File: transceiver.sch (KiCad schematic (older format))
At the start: 1 part, among them U3 CC1200

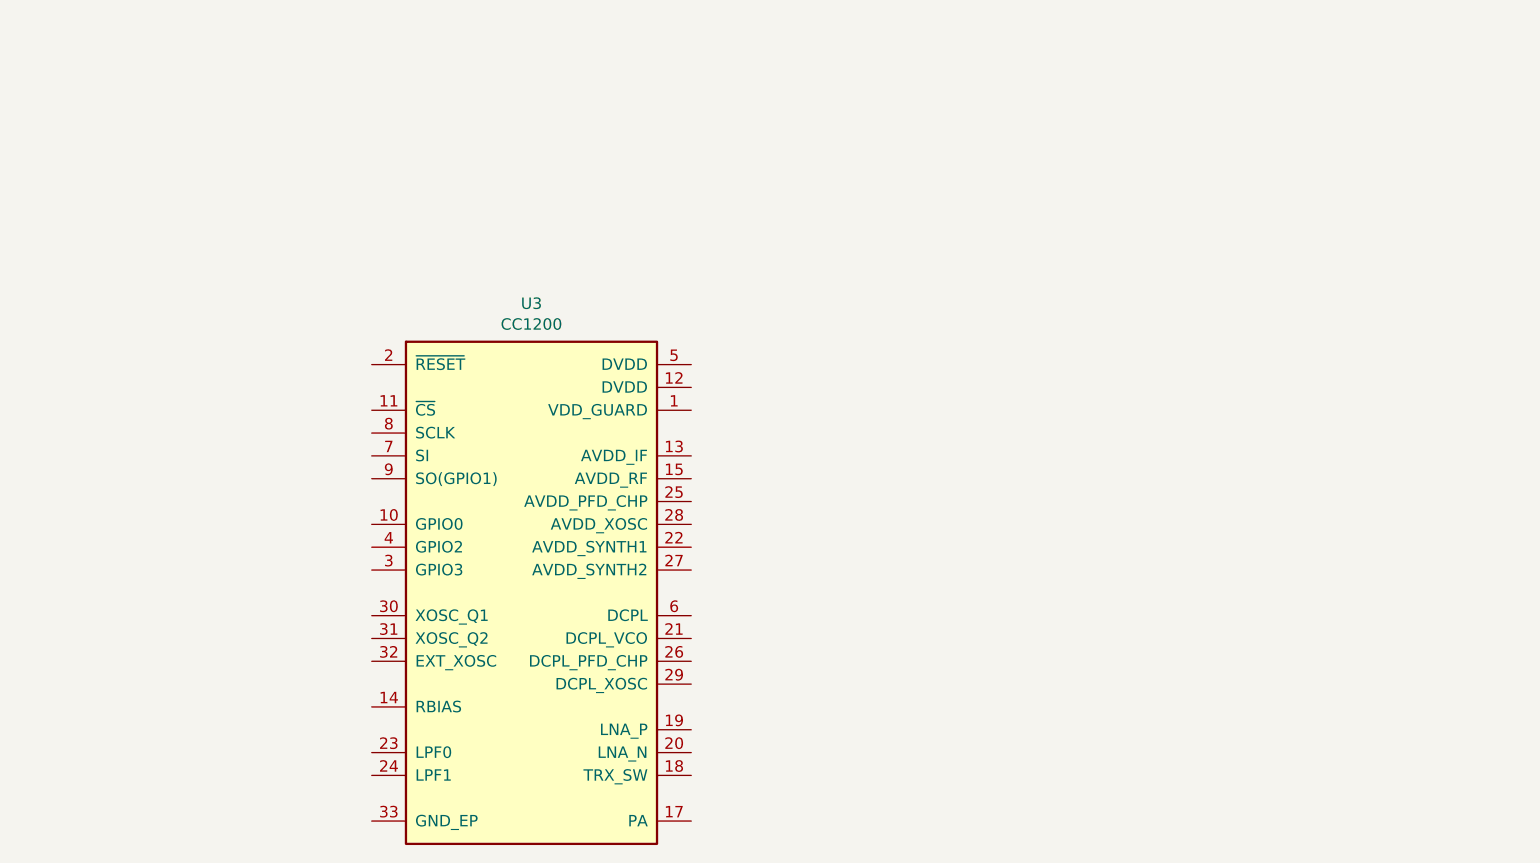
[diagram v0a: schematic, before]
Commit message: Started work on CC1200
might not be actual final tranciever
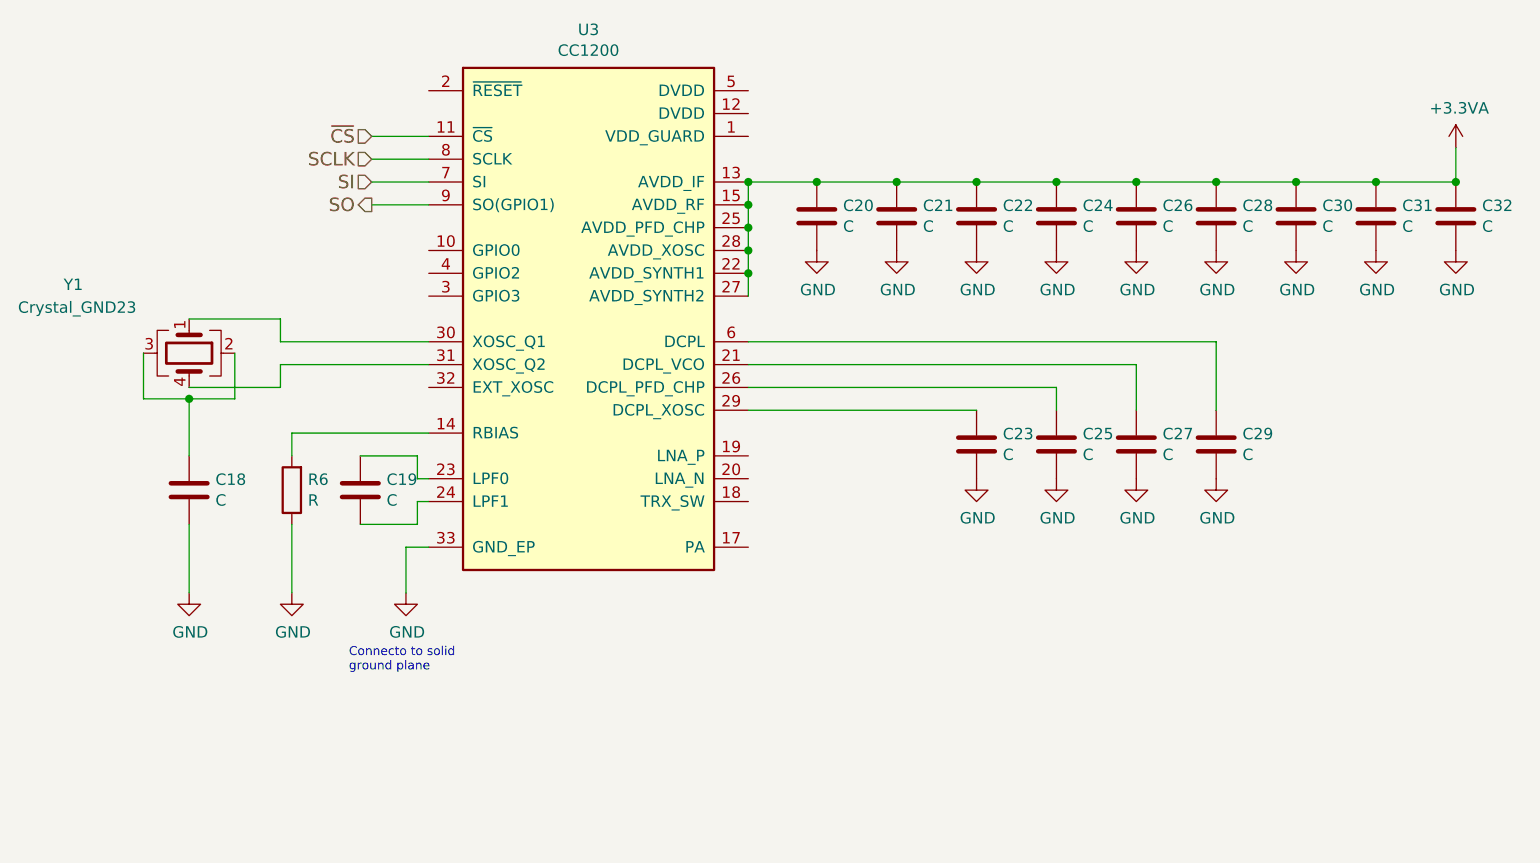
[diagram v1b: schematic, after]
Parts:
- added C18, C19, C20, C21, C22, C23, C24, C25, C26, C27, C28, C29, C30, C31, C32: C, symbol Device:C
- added R6: R, symbol Device:R
- added Y1: Crystal_GND23, symbol Device:Crystal_GND23
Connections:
- net ~CS: now reaches U3.11 (~CS~)
- net +3.3VA: now reaches U3.13 (AVDD_IF)
- net +3.3VA: now also U3.15 (AVDD_RF), U3.22 (AVDD_SYNTH1), U3.25 (AVDD_PFD_CHP), U3.27 (AVDD_SYNTH2), U3.28 (AVDD_XOSC), C20.1, C21.1, C22.1, C24.1, C26.1, C28.1, C30.1, C31.1, C32.1
- net at U3.14 (RBIAS): now also R6.2
- net at U3.21 (DCPL_VCO): now also C27.1
- net at U3.23 (LPF0): now also C19.1
- net at U3.24 (LPF1): now also C19.2
- net at U3.26 (DCPL_PFD_CHP): now also C25.1
- net at U3.29 (DCPL_XOSC): now also C23.1
- net at U3.30 (XOSC_Q1): now also Y1.1
- net at U3.31 (XOSC_Q2): now also Y1.4
- net GND: now reaches U3.33 (GND_EP)
- net GND: now also C18.2, C20.2, C21.2, C22.2, C23.2, C24.2, C25.2, C26.2, C27.2, C28.2, C29.2, C30.2, C31.2, C32.2, R6.1
- net at U3.6 (DCPL): now also C29.1
- net SI: now reaches U3.7 (SI)
- net SCLK: now reaches U3.8 (SCLK)
- net SO: now reaches U3.9 (SO(GPIO1))
- new net: C18.1, Y1.2, Y1.3
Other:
- note added: "Connecto to solid \nground plane\n"
- moved on the sheet: U3
